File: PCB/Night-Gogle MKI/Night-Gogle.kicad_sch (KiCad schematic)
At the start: 0 parts

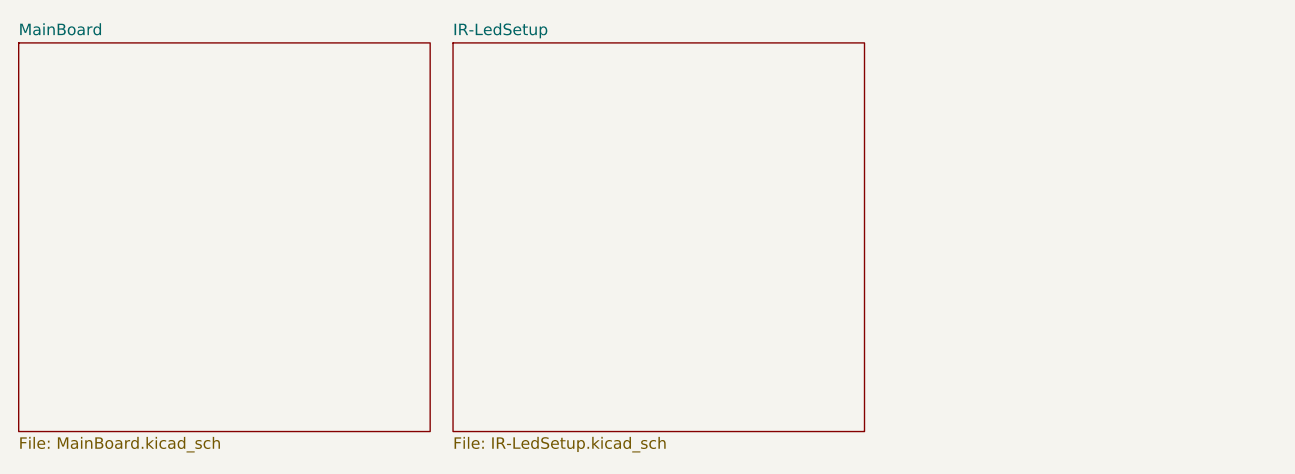
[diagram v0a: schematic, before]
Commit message: pcb update
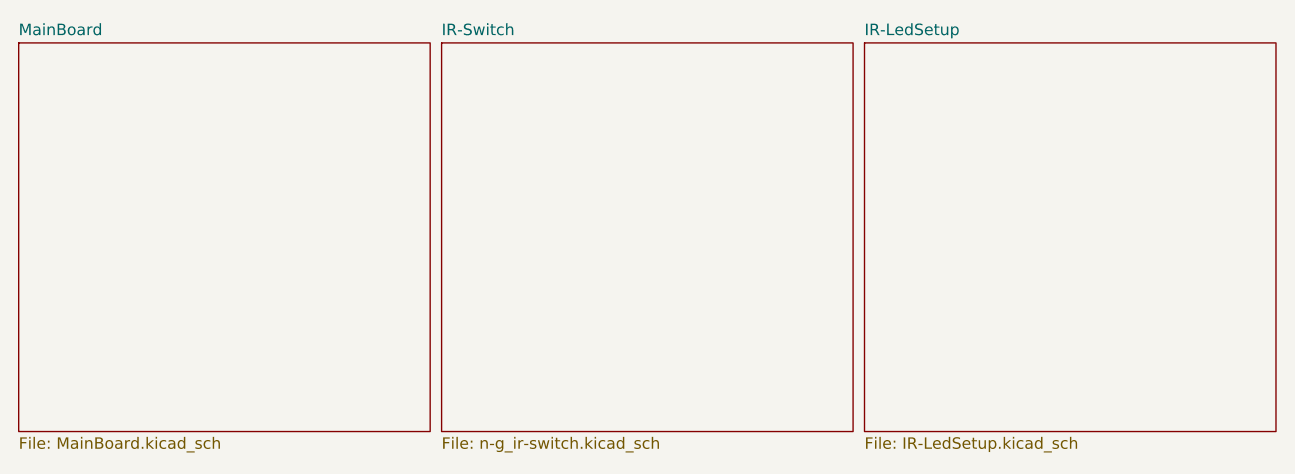
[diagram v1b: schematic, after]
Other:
- added sheet IR-Switch (n-g_ir-switch.kicad_sch)
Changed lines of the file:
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@@
 	(paper "A4")
 	(sheet
-		(at 62.23 15.24)
+		(at 60.96 15.24)
+		(size 45.72 43.18)
+		(exclude_from_sim no)
+		(in_bom yes)
+		(on_board yes)
+		(dnp no)
+		(fields_autoplaced yes)
+		(stroke
+			(width 0.1524)
+			(type solid)
+		)
+		(fill
+			(color 0 0 0 0.0000)
+		)
+		(property "Sheetname" "IR-Switch"
+			(at 60.96 14.5284 0)
+			(effects
+				(font
+					(size 1.27 1.27)
+				)
+				(justify left bottom)
+			)
+		)
+		(property "Sheetfile" "n-g_ir-switch.kicad_sch"
+			(at 60.96 59.0046 0)
+			(effects
+				(font
+					(size 1.27 1.27)
+				)
+				(justify left top)
+			)
+		)
+		(instances
+			(project "Night-Gogle"
+				(path "/46563032-f0f5-44cd-9207-962e2cbfd880"
+					(page "3")
+				)
+			)
+		)
+	)
+	(sheet
+		(at 107.95 15.24)
 		(size 45.72 43.18)
 		(exclude_from_sim no)
@@
 		)
 		(property "Sheetname" "IR-LedSetup"
-			(at 62.23 14.5284 0)
+			(at 107.95 14.5284 0)
 			(effects
 				(font
@@
 		)
 		(property "Sheetfile" "IR-LedSetup.kicad_sch"
-			(at 62.23 59.0046 0)
+			(at 107.95 59.0046 0)
 			(effects
 				(font
@@
 			(project "Night-Gogle"
 				(path "/46563032-f0f5-44cd-9207-962e2cbfd880"
-					(page "3")
+					(page "4")
 				)
 			)
